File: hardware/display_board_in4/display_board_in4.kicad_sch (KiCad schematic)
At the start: 142 parts, among them J1 Conn_02x05_Odd_Even, J3 Conn_02x05_Odd_Even, Q1 MMBTA42, Q10 MMBTA42, Q11 MMBTA42, Q12 MMBTA42, Q13 MMBTA42, Q14 MMBTA42, Q15 MMBTA42, Q16 MMBTA42, Q17 MMBTA42, Q18 MMBTA42, Q19 MMBTA42, Q2 MMBTA42, Q20 MMBTA42, Q21 MMBTA42, Q22 MMBTA42, Q23 MMBTA42, Q24 MMBTA42, Q25 MMBTA42, Q26 MMBTA42, Q27 MMBTA42, Q28 MMBTA42, Q29 MMBTA42, Q3 MMBTA42, Q30 MMBTA42, Q31 MMBTA42, Q32 MMBTA42, Q33 MMBTA42, Q34 MMBTA42, Q35 MMBTA42, Q36 MMBTA42, Q37 MMBTA42, Q38 MMBTA42, Q39 MMBTA42, Q4 MMBTA42, Q40 MMBTA42, Q41 MMBTA42, Q42 MMBTA42, Q43 MMBTA42, Q44 MMBTA42, Q45 MMBTA42, Q46 MMBTA42, Q47 MMBTA42, Q48 MMBTA42, Q49 MMBTA42, Q5 MMBTA42, Q50 MMBTA42, Q51 MMBTA42, Q52 MMBTA42, Q53 MMBTA42, Q54 MMBTA42, Q55 MMBTA42, Q56 MMBTA42, Q57 MMBTA42, Q58 MMBTA42, Q59 MMBTA42, Q6 MMBTA42, Q60 MMBTA42, Q7 MMBTA42, Q8 MMBTA42, Q9 MMBTA42, SW1 XKB5858-W-E-75, U1 PCA9685PW, U2 PCA9685PW, U3 PCA9685PW, U4 PCA9685PW, U5 LTR-303ALS-01

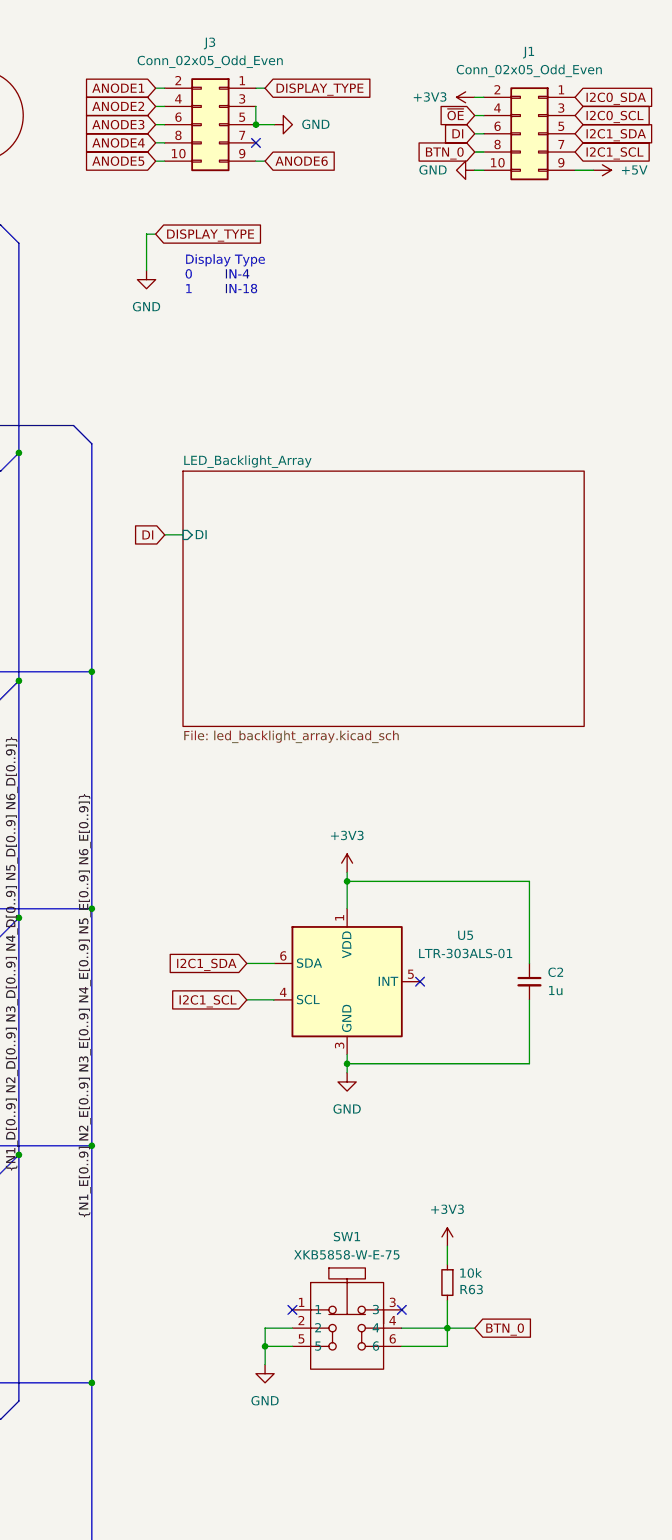
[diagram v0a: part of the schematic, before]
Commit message: WIP: schematic and layout
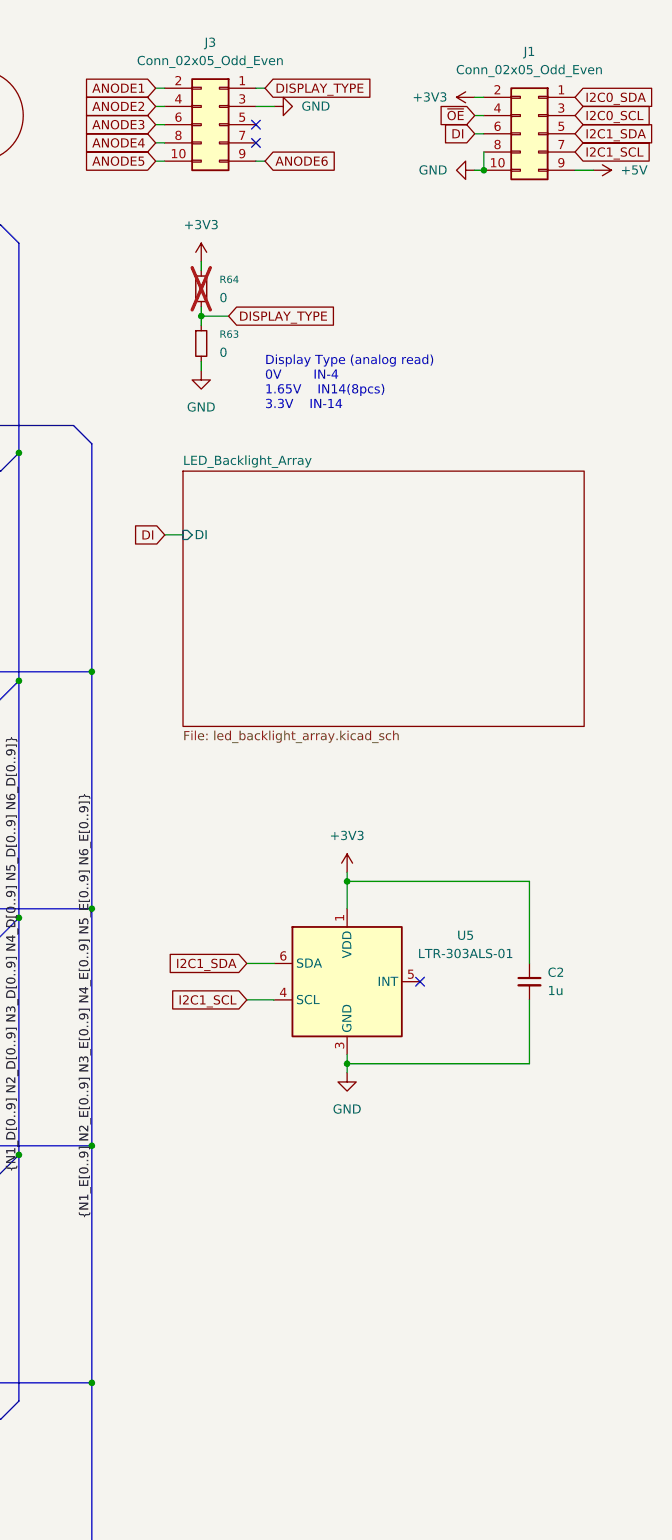
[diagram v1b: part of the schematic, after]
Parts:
- removed SW1: XKB5858-W-E-75, habonroof_kicad_library:XKB5858, symbol Johnson_Symbol_Lib:SW_push_RightAngle
- added R64: 0, Resistor_SMD:R_0603_1608Metric, symbol Device:R_Small
- R63: value 10k -> 0; footprint Resistor_SMD:R_0402_1005Metric -> Resistor_SMD:R_0603_1608Metric; LCSC PN C25744 -> (none)
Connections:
- net BTN_0 is gone; now on net GND: J1.8 (Pin_8), R63.2
- net +3V3: now also R64.1; no longer R63.1
- net GND: no longer J3.1 (Pin_1), J3.5 (Pin_5)
- new net DISPLAY_TYPE: J3.1 (Pin_1), R63.1, R64.2
- no-connect marks 8 -> 7
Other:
- note added: "Display Type (analog read) 0V IN-4 1.65V IN14(8pcs) 3.3V IN-14"
- note removed: "Display Type 0 IN-4 1 IN-18"
